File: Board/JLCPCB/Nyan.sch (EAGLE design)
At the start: 63 parts, among them IC1 74HCT541PW, IC2 STM32F10XCXT6, IC3 74HCT541PW, IC4 ST3485, U2 A4988_STEP, U3 MAX6966, X1 WR-WTB2.0-2_THT-VER, X10 32768, X2 WR-WTB2.0-4_THT_VER, X3 WR-WTB2.0-5_THT-VER, X4 WR-WTB2.0-5_THT-VER, X6 68610614122, X7 68612414422, X8 68610414122, X9 8M

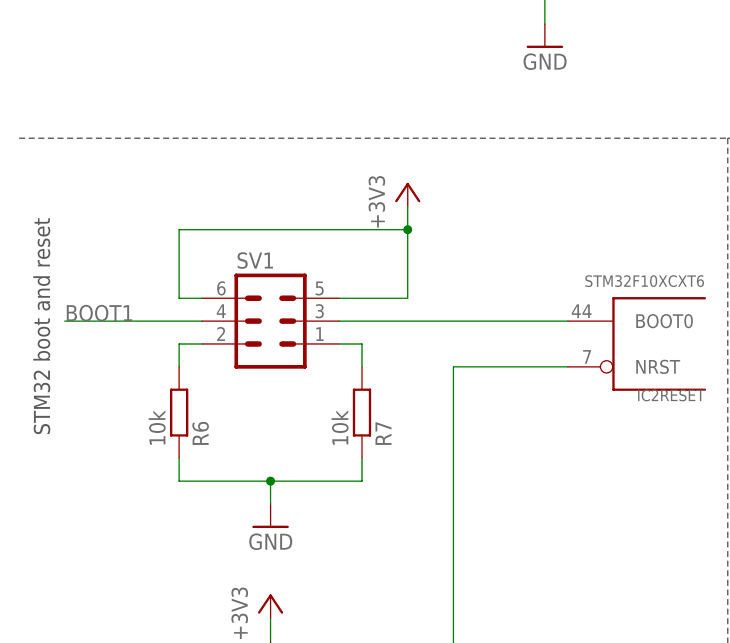
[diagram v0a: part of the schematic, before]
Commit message: [Board] A little more layouting done
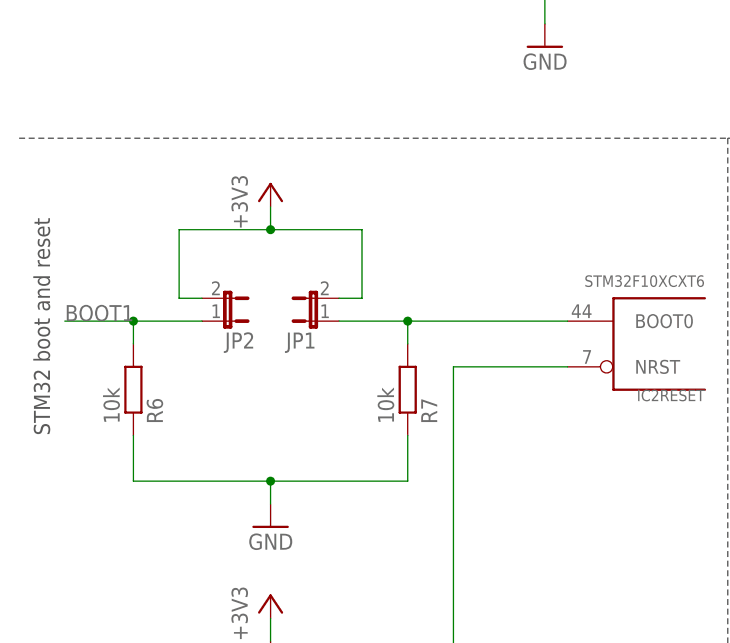
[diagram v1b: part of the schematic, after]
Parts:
- removed SV1: (no value), con-lstb:MA03-2
- added JP1, JP2: (no value), jumper:JP1E
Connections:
- removed net N$12: R6.2, SV1.2
- removed net N$13: R7.2, SV1.1
- net +3V3: now also JP1.2, JP2.2; no longer SV1.5, SV1.6
- net BOOT1: now also JP2.1, R6.2; no longer SV1.4
- net N$7: now also JP1.1, R7.2; no longer SV1.3
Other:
- moved on the sheet: R6, R7
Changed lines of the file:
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@@
 <part name="SJ1" library="jumper" deviceset="SJ2W" device=""/>
 <part name="SJ2" library="jumper" deviceset="SJ2W" device=""/>
-<part name="SV1" library="con-lstb" deviceset="MA03-2" device=""/>
 <part name="+3V6" library="supply1" deviceset="+3V3" device=""/>
 <part name="R6" library="rcl" deviceset="R-EU_" device="R0603" value="10k"/>
@@
 <part name="C21" library="rcl" deviceset="C-EU" device="C0603" value="1u"/>
 <part name="X3" library="TURAG_Steckverbinder" deviceset="WR-WTB2.0-5" device="_THT-VER"/>
+<part name="JP1" library="jumper" deviceset="JP1E" device=""/>
+<part name="JP2" library="jumper" deviceset="JP1E" device=""/>
 </parts>
 <sheets>
@@
 <instance part="SJ1" gate="G$1" x="40.64" y="30.48" rot="R90"/>
 <instance part="SJ2" gate="G$1" x="40.64" y="12.7" rot="R270"/>
-<instance part="SV1" gate="1" x="27.94" y="-88.9"/>
-<instance part="+3V6" gate="G$1" x="43.18" y="-73.66"/>
-<instance part="R6" gate="G$1" x="17.78" y="-99.06" rot="MR90"/>
-<instance part="R7" gate="G$1" x="38.1" y="-99.06" rot="MR90"/>
+<instance part="+3V6" gate="G$1" x="27.94" y="-73.66"/>
+<instance part="R6" gate="G$1" x="12.7" y="-96.52" rot="MR90"/>
+<instance part="R7" gate="G$1" x="43.18" y="-96.52" rot="MR90"/>
 <instance part="GND15" gate="1" x="58.42" y="-58.42" rot="MR0"/>
 <instance part="GND16" gate="1" x="27.94" y="-111.76" rot="MR0"/>
@@
 <instance part="C21" gate="G$1" x="27.94" y="-43.18" rot="MR180"/>
 <instance part="X3" gate="G$1" x="33.02" y="73.66" rot="R180"/>
+<instance part="JP1" gate="A" x="33.02" y="-88.9" rot="R90"/>
+<instance part="JP2" gate="A" x="22.86" y="-88.9" rot="MR90"/>
 </instances>
 <busses>
@@
 <segment>
 <pinref part="R6" gate="G$1" pin="1"/>
-<wire x1="17.78" y1="-104.14" x2="17.78" y2="-106.68" width="0.1524" layer="91"/>
-<wire x1="17.78" y1="-106.68" x2="27.94" y2="-106.68" width="0.1524" layer="91"/>
+<wire x1="12.7" y1="-101.6" x2="12.7" y2="-106.68" width="0.1524" layer="91"/>
 <pinref part="GND16" gate="1" pin="GND"/>
+<wire x1="12.7" y1="-106.68" x2="27.94" y2="-106.68" width="0.1524" layer="91"/>
 <wire x1="27.94" y1="-106.68" x2="27.94" y2="-109.22" width="0.1524" layer="91"/>
 <pinref part="R7" gate="G$1" pin="1"/>
-<wire x1="27.94" y1="-106.68" x2="38.1" y2="-106.68" width="0.1524" layer="91"/>
-<wire x1="38.1" y1="-106.68" x2="38.1" y2="-104.14" width="0.1524" layer="91"/>
+<wire x1="27.94" y1="-106.68" x2="43.18" y2="-106.68" width="0.1524" layer="91"/>
+<wire x1="43.18" y1="-106.68" x2="43.18" y2="-101.6" width="0.1524" layer="91"/>
 <junction x="27.94" y="-106.68"/>
 </segment>
@@
 </segment>
 <segment>
-<pinref part="SV1" gate="1" pin="5"/>
-<wire x1="35.56" y1="-86.36" x2="43.18" y2="-86.36" width="0.1524" layer="91"/>
-<wire x1="43.18" y1="-86.36" x2="43.18" y2="-78.74" width="0.1524" layer="91"/>
-<pinref part="SV1" gate="1" pin="6"/>
-<wire x1="43.18" y1="-78.74" x2="43.18" y2="-76.2" width="0.1524" layer="91"/>
-<wire x1="20.32" y1="-86.36" x2="17.78" y2="-86.36" width="0.1524" layer="91"/>
-<wire x1="17.78" y1="-86.36" x2="17.78" y2="-78.74" width="0.1524" layer="91"/>
-<wire x1="17.78" y1="-78.74" x2="43.18" y2="-78.74" width="0.1524" layer="91"/>
-<junction x="43.18" y="-78.74"/>
-<pinref part="+3V6" gate="G$1" pin="+3V3"/>
-</segment>
-<segment>
 <pinref part="R8" gate="G$1" pin="2"/>
 <pinref part="+3V7" gate="G$1" pin="+3V3"/>
@@
 <pinref part="+3V1" gate="G$1" pin="+3V3"/>
 </segment>
+<segment>
+<wire x1="35.56" y1="-86.36" x2="38.1" y2="-86.36" width="0.1524" layer="91"/>
+<wire x1="38.1" y1="-86.36" x2="38.1" y2="-78.74" width="0.1524" layer="91"/>
+<wire x1="20.32" y1="-86.36" x2="17.78" y2="-86.36" width="0.1524" layer="91"/>
+<wire x1="17.78" y1="-86.36" x2="17.78" y2="-78.74" width="0.1524" layer="91"/>
+<wire x1="17.78" y1="-78.74" x2="27.94" y2="-78.74" width="0.1524" layer="91"/>
+<pinref part="JP1" gate="A" pin="2"/>
+<pinref part="JP2" gate="A" pin="2"/>
+<pinref part="+3V6" gate="G$1" pin="+3V3"/>
+<wire x1="27.94" y1="-78.74" x2="38.1" y2="-78.74" width="0.1524" layer="91"/>
+<wire x1="27.94" y1="-76.2" x2="27.94" y2="-78.74" width="0.1524" layer="91"/>
+<junction x="27.94" y="-78.74"/>
+</segment>
 </net>
 <net name="M2B" class="0">
@@
 </segment>
 <segment>
-<pinref part="SV1" gate="1" pin="4"/>
-<wire x1="20.32" y1="-88.9" x2="5.08" y2="-88.9" width="0.1524" layer="91"/>
+<wire x1="20.32" y1="-88.9" x2="12.7" y2="-88.9" width="0.1524" layer="91"/>
 <label x="5.08" y="-88.9" size="1.778" layer="95"/>
+<pinref part="R6" gate="G$1" pin="2"/>
+<wire x1="12.7" y1="-88.9" x2="5.08" y2="-88.9" width="0.1524" layer="91"/>
+<wire x1="12.7" y1="-91.44" x2="12.7" y2="-88.9" width="0.1524" layer="91"/>
+<junction x="12.7" y="-88.9"/>
+<pinref part="JP2" gate="A" pin="1"/>
 </segment>
 </net>
 <net name="N$7" class="0">
 <segment>
-<pinref part="SV1" gate="1" pin="3"/>
 <pinref part="IC2" gate="RESET" pin="BOOT0"/>
-<wire x1="35.56" y1="-88.9" x2="60.96" y2="-88.9" width="0.1524" layer="91"/>
-</segment>
-</net>
-<net name="N$12" class="0">
-<segment>
-<pinref part="R6" gate="G$1" pin="2"/>
-<pinref part="SV1" gate="1" pin="2"/>
-<wire x1="17.78" y1="-93.98" x2="17.78" y2="-91.44" width="0.1524" layer="91"/>
-<wire x1="17.78" y1="-91.44" x2="20.32" y2="-91.44" width="0.1524" layer="91"/>
-</segment>
-</net>
-<net name="N$13" class="0">
-<segment>
-<pinref part="SV1" gate="1" pin="1"/>
+<wire x1="35.56" y1="-88.9" x2="43.18" y2="-88.9" width="0.1524" layer="91"/>
 <pinref part="R7" gate="G$1" pin="2"/>
-<wire x1="35.56" y1="-91.44" x2="38.1" y2="-91.44" width="0.1524" layer="91"/>
-<wire x1="38.1" y1="-91.44" x2="38.1" y2="-93.98" width="0.1524" layer="91"/>
-</segment>
-</net>
+<wire x1="43.18" y1="-88.9" x2="60.96" y2="-88.9" width="0.1524" layer="91"/>
+<wire x1="43.18" y1="-91.44" x2="43.18" y2="-88.9" width="0.1524" layer="91"/>
+<junction x="43.18" y="-88.9"/>
+<pinref part="JP1" gate="A" pin="1"/>
+</segment>
+</net>
